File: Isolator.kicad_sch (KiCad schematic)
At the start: 12 parts, among them U11 EL817, U16 EL817, U17 EL817, U8 EL817

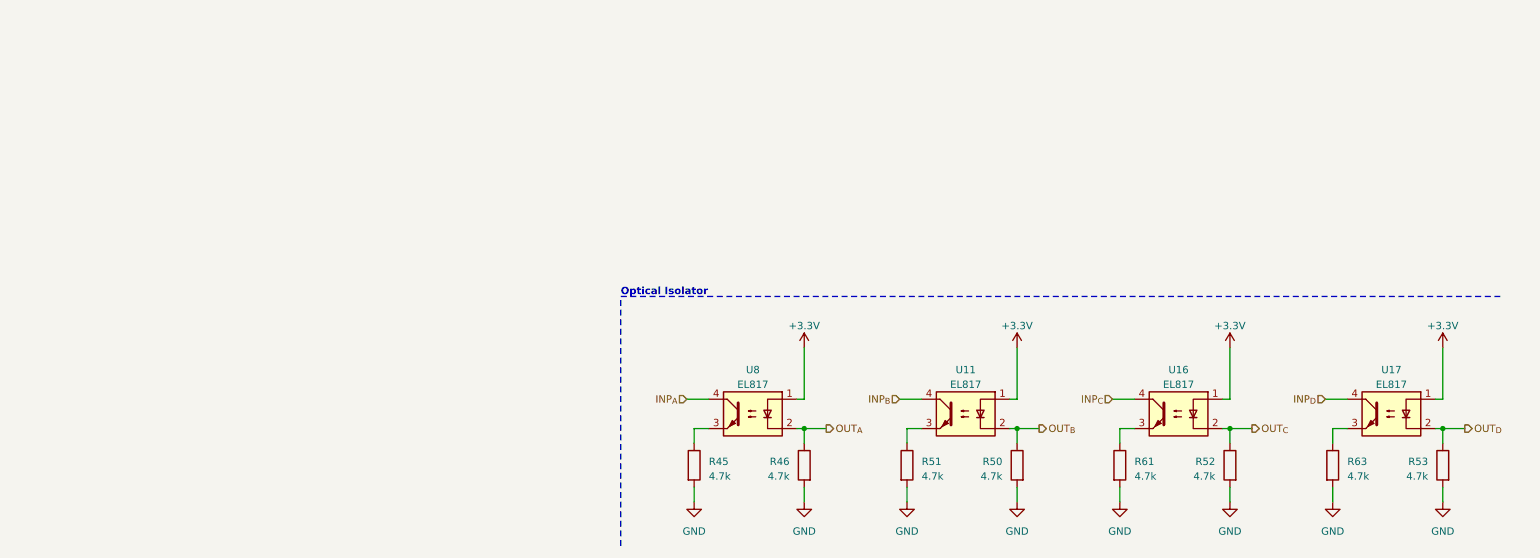
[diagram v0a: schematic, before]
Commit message: Battery Managment System V1.0
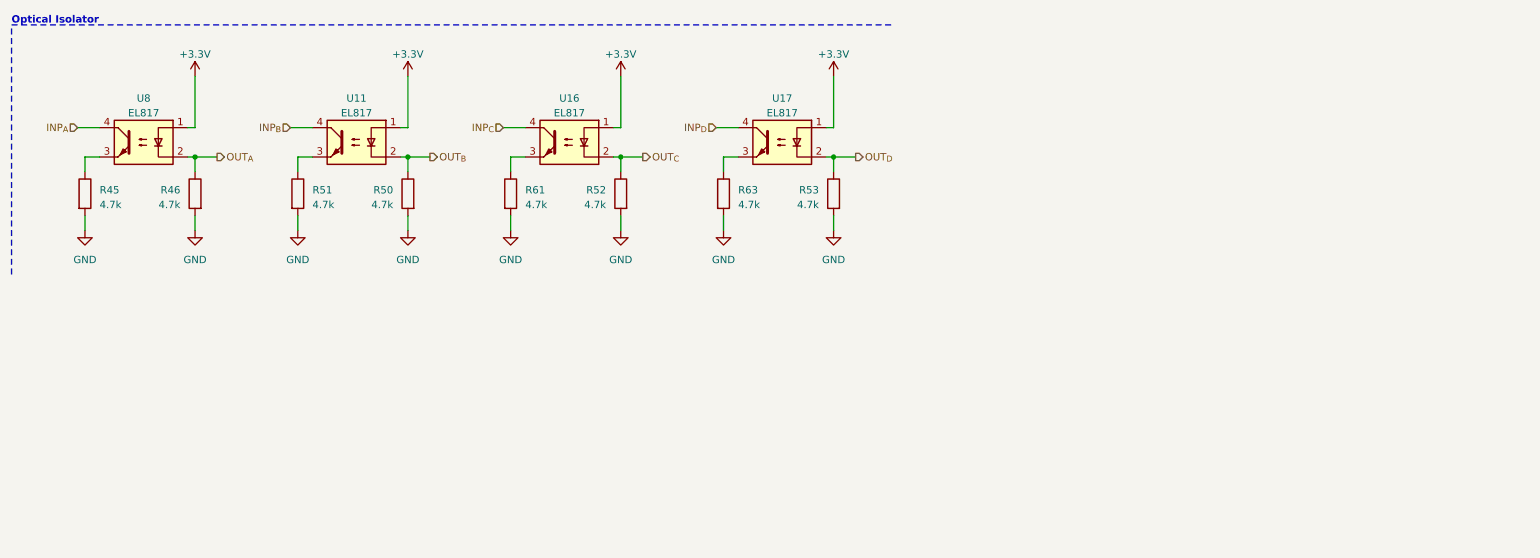
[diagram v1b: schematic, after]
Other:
- moved on the sheet: R45, R46, R50, R51, R52, R53, R61, R63, U11, U16, U17, U8
